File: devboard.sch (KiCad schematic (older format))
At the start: 7 parts, among them J1 USB_B

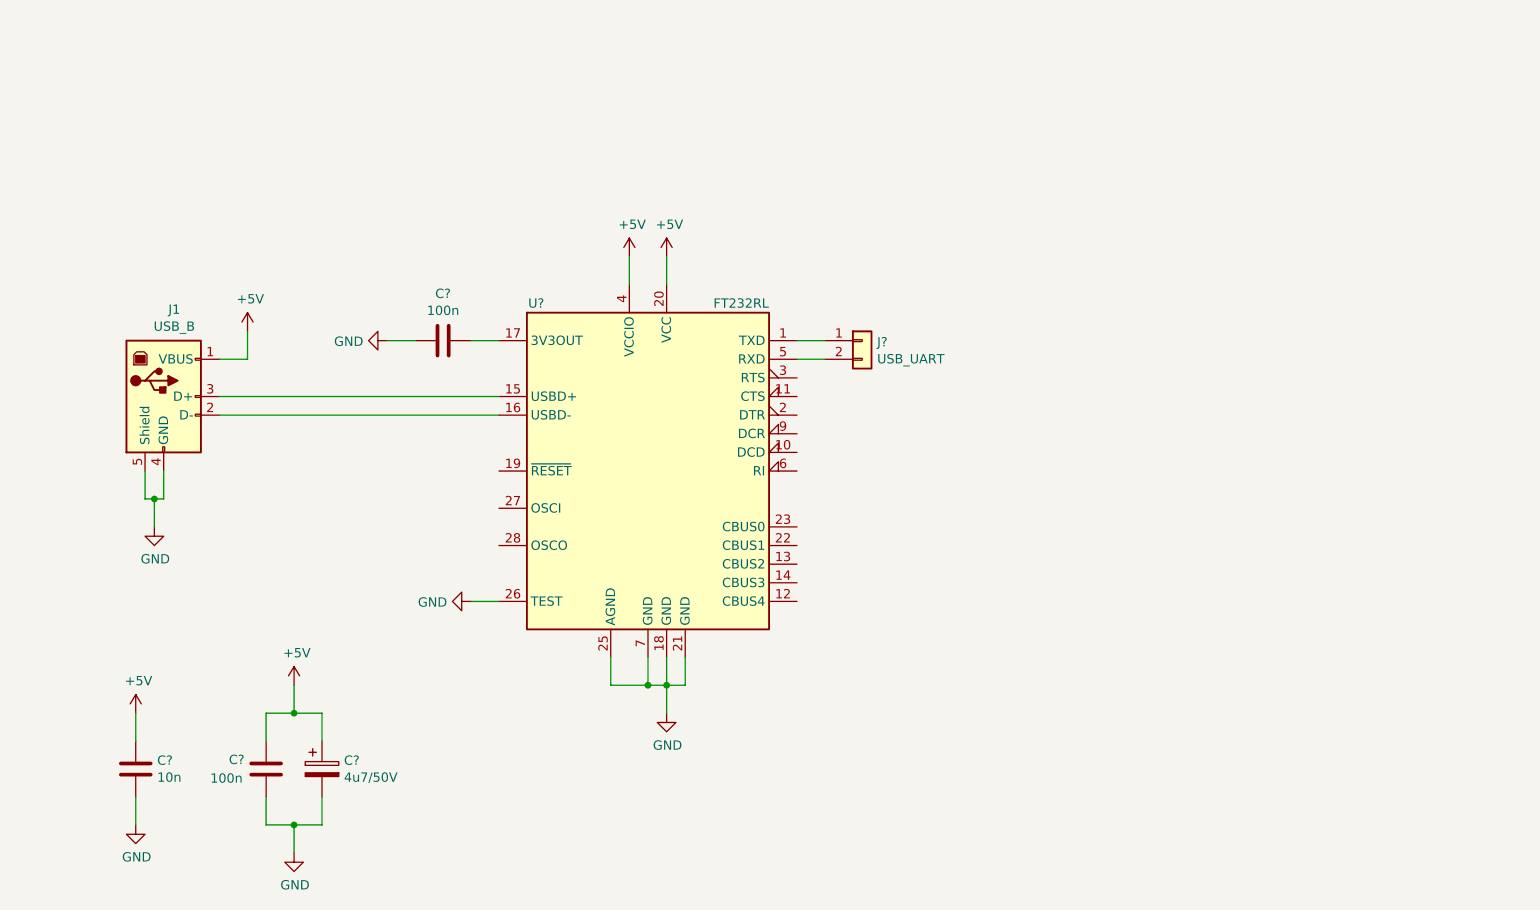
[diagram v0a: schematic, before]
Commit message: power dokończony essa
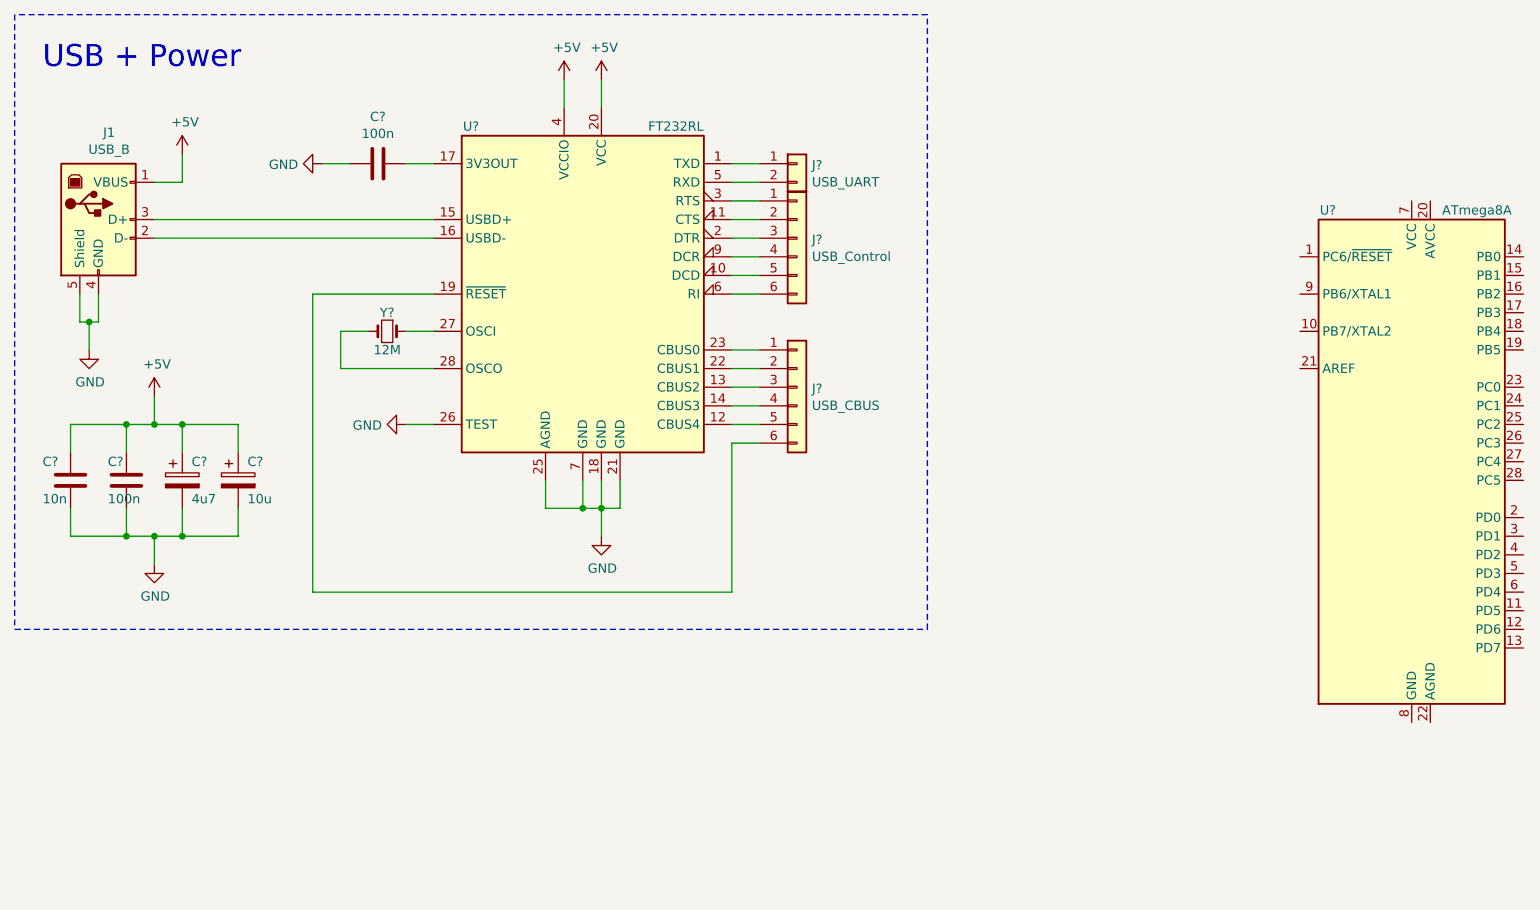
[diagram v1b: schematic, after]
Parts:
- added C?: 10u, symbol Device:CP
- added J?: USB_Control, symbol Connector_Generic:Conn_01x06
- added J?: USB_CBUS, symbol Connector_Generic:Conn_01x06
- added U?: ATmega8A, Package_DIP:DIP-28_W7.62mm, symbol MCU_Microchip_ATmega:ATmega8A-PU
- added Y?: 12M, symbol Device:Crystal_Small
- C?: value 4u7/50V -> 4u7
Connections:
- net +5V: now also C?.1
- net GND: now also C?.2
- net at U?.10 (DCD): now also J?.5 (Pin_5)
- net at U?.11 (CTS): now also J?.2 (Pin_2)
- net at U?.12 (CBUS4): now also J?.5 (Pin_5)
- net at U?.13 (CBUS2): now also J?.3 (Pin_3)
- net at U?.14 (CBUS3): now also J?.4 (Pin_4)
- net at U?.19 (~RESET~): now also J?.6 (Pin_6)
- net at U?.2 (DTR): now also J?.3 (Pin_3)
- net at U?.22 (CBUS1): now also J?.2 (Pin_2)
- net at U?.23 (CBUS0): now also J?.1 (Pin_1)
- net at U?.27 (OSCI): now also Y?.1
- net at U?.28 (OSCO): now also Y?.2
- net at U?.3 (RTS): now also J?.1 (Pin_1)
- net at U?.6 (RI): now also J?.6 (Pin_6)
- net at U?.9 (DCR): now also J?.4 (Pin_4)
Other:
- note added: "USB + Power"
- moved on the sheet: C?, J1, J?, U?
